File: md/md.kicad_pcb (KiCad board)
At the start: 2 copper layers, 49.5 x 66 mm, 51 parts, among them J1 OutB, J2 OutA, J3 Conn_01x04, J4 GS2, J5 Conn_02x08_Counter_Clockwise, J6 Conn_02x08_Counter_Clockwise, J7 Conn_02x08_Counter_Clockwise, J8 Conn_02x08_Counter_Clockwise, Q1 IRFB7437PBF, Q2 IRFB7437PBF, Q3 IRFB7437PBF, Q4 IRFB7437PBF, U1 TLP2105, U2 IRS2302, U3 IRS2302, U4 7400, U5 L7812

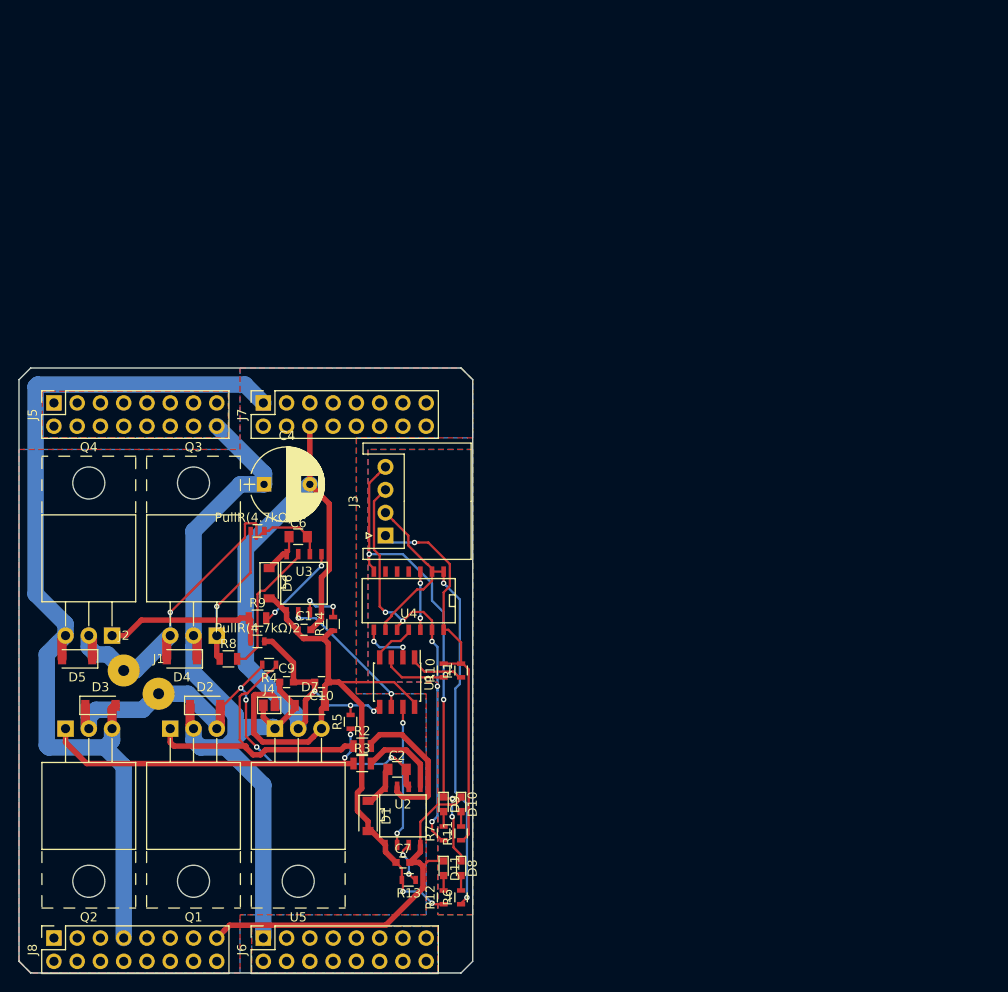
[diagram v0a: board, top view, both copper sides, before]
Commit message: だいたい配置出来た
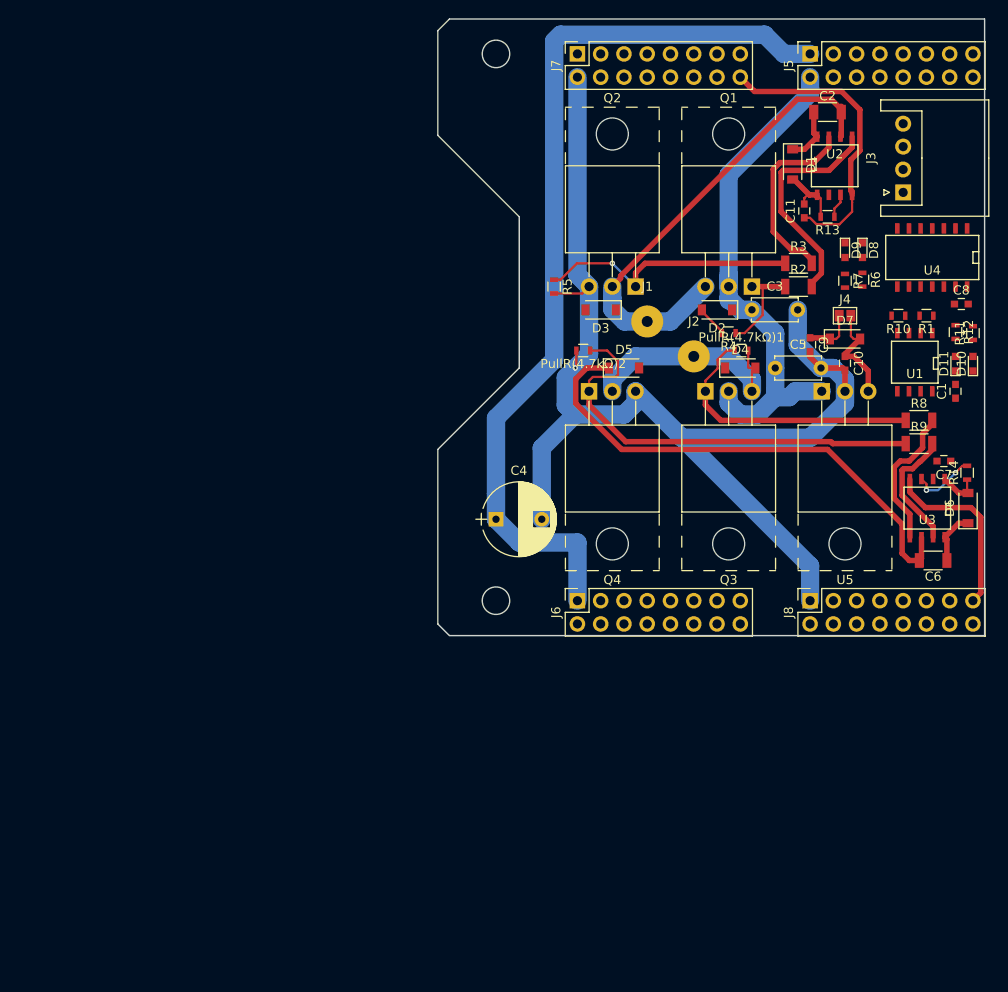
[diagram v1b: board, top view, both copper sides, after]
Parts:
- added C11: C, Capacitors_SMD:C_0603, F.Cu at (212.7, 78.1)
- added C3: PowerC, Capacitors_THT:C_Disc_D5.0mm_W2.5mm_P5.00mm, F.Cu at (207.0, 88.9)
- added C5: PowerC, Capacitors_THT:C_Disc_D5.0mm_W2.5mm_P5.00mm, F.Cu at (209.6, 95.2)
- added C8: C, Capacitors_SMD:C_0603, F.Cu at (229.9, 88.3)
- C10: value 1uF -> RegOutC(1uF)
- C2, C6: value 10uF -> BootC(10uF); footprint Capacitors_SMD:C_0805 -> Capacitors_SMD:C_1206
- C4: value CP -> PowerCP
- C9: value 1uF -> RegInC(1uF)
- D10: value SML-E12P8T86 -> 5VLED(SML-E12P8T86)
- D11: value SML-E12V8WT86 -> 12VLED(SML-E12V8WT86)
- D2, D3, D4, D5: value SS2040FL -> RevD(SS2040FL)
- D7: value SS2040FL -> RegRevC(SS2040FL)
- D8: value SML-E12Y8WT86 -> DIRLED(SML-E12Y8WT86)
- D9: value SML-E13BC8TT86 -> LED(SML-E13BC8TT86)
- J3: value Conn_01x04 -> Interface
- J4: value GS2 -> 12VJmp
- Q1, Q2: value IRFB7437PBF -> FETA(IRFB7437PBF)
- Q3, Q4: value IRFB7437PBF -> FETB(IRFB7437PBF)
- R11: value LEDR(470Ω) -> 5VLEDR(470Ω)
- R12: value LEDR(1.2kΩ) -> 12VLEDR(1.2kΩ)
- R14: value R -> PullR
- R2, R3, R8, R9: value GateR(6.8Ω) -> GateR(8.2Ω); footprint Resistors_SMD:R_0805 -> Resistors_SMD:R_1206
- R6: value LEDR(470Ω) -> DIRLEDR(470Ω)
- R7: value LEDR(470Ω) -> PWMLEDR(470Ω)
- U1: footprint Housings_SOIC:SOIC-8_3.9x4.9mm_Pitch1.27mm -> SMD_Packages:SOIC-8-N
- U2, U3: value IRS2302 -> IR7184S
- moved J5 90.9 mm to (213.4, 61.0)
- moved J8 90.4 mm to (213.4, 120.7)
- moved C2 85.8 mm to (215.3, 67.3)
- moved R13 85.6 mm to (215.3, 78.7)
- moved U2 85.2 mm to (216.0, 73.2)
- moved D1 84.9 mm to (211.5, 73.0)
- moved R12 83.3 mm to (229.2, 91.3), turned to 270 degrees
- moved D8 80.5 mm to (219.1, 82.4)
- moved R6 80.4 mm to (219.1, 85.6), turned to 270 degrees
- moved Q1 79.8 mm to (207.0, 86.4), turned to 180 degrees
- moved R8 79.8 mm to (225.2, 101.0)
- moved Q2 78.8 mm to (194.3, 86.4), turned to 180 degrees
- moved D11 78.5 mm to (229.2, 94.8), turned to 90 degrees
- moved R11 78.1 mm to (231.1, 91.4)
- moved D6 76.7 mm to (230.6, 110.5), turned to 90 degrees
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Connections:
- J3 pad 1: +5V -> GND
- J3 pad 2: /DIR -> +5V
- J3 pad 4: GND -> /DIR
- U2 pad 5: Net-(R3-Pad2) -> Net-(R2-Pad2)
- U2 pad 7: Net-(R2-Pad2) -> Net-(R3-Pad2)
- U3 pad 5: Net-(R9-Pad2) -> Net-(R8-Pad2)
- U3 pad 7: Net-(R8-Pad2) -> Net-(R9-Pad2)
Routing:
- net +24V: track 91.9 -> 161.8 mm
- net /DIR: track 56.7 -> 0.00 mm, vias 2 -> 0
- net +12V: track 79.3 -> 23.7 mm, vias 2 -> 0
- net GND: track 52.7 -> 0.00 mm, vias 4 -> 0
- net /PWM: track 48.2 -> 0.00 mm, vias 5 -> 0
- net +5V: track 42.6 -> 0.00 mm, vias 1 -> 0
- net Net-(C6-Pad2): track 45.3 -> 81.1 mm, vias 1 -> 0
- net GNDPWR: track 224.4 -> 188.7 mm, vias 3 -> 1
- net Net-(PullR(4.7kΩ)2-Pad1): track 18.3 -> 47.4 mm
- net Net-(Q1-Pad1): track 33.8 -> 11.7 mm
- net /OUTB: track 15.6 -> 0.00 mm, vias 2 -> 0
- net /OUTA: track 15.3 -> 0.00 mm, vias 2 -> 0
- net Net-(PullR(4.7kΩ)1-Pad1): track 15.6 -> 30.3 mm, vias 1 -> 0
- net Net-(R3-Pad2): track 9.14 -> 20.9 mm
- net Net-(Q2-Pad1): track 38.0 -> 28.9 mm, vias 2 -> 1
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- removed copper zone on B.Cu, net +24V
- removed copper zone on F.Cu, net +24V
- removed copper zone on B.Cu, net GND
- removed copper zone on F.Cu, net GND
- removed copper zone on B.Cu, net GNDPWR
- removed copper zone on F.Cu, net GNDPWR
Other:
- board size 49.5 x 66 mm -> 59.7 x 67.3 mm
